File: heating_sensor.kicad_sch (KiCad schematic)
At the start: 3 parts

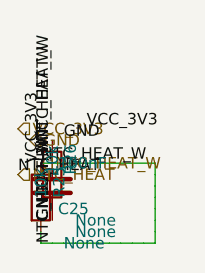
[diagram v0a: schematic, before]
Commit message: fix writer
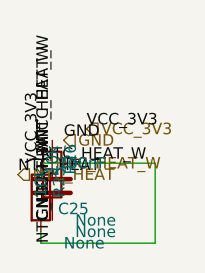
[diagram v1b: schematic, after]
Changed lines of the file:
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@@
 		(instances
 			(project "Untitled"
-				(path "/51987713-8abd-43cc-8dc0-832c464dab57"
+				(path "/c49ef74a-788a-4bab-9f15-e22212d1716d"
 					(reference "C25")
 					(unit 1)
@@
 		(instances
 			(project "Untitled"
-				(path "/51987713-8abd-43cc-8dc0-832c464dab57"
+				(path "/c49ef74a-788a-4bab-9f15-e22212d1716d"
 					(reference "R25")
 					(unit 1)
@@
 		(instances
 			(project "Untitled"
-				(path "/51987713-8abd-43cc-8dc0-832c464dab57"
+				(path "/c49ef74a-788a-4bab-9f15-e22212d1716d"
 					(reference "R26")
 					(unit 1)
@@
 	(wire
 		(pts
-			(xy 16.51 24.13) (xy 17.78 24.13)
-		)
-		(stroke
-			(width 0)
-			(type default)
-		)
-	)
-	(wire
-		(pts
-			(xy 17.78 24.13) (xy 19.05 24.13)
-		)
-		(stroke
-			(width 0)
-			(type default)
-		)
-	)
-	(wire
-		(pts
-			(xy 19.05 24.13) (xy 20.32 24.13)
-		)
-		(stroke
-			(width 0)
-			(type default)
-		)
-	)
-	(wire
-		(pts
-			(xy 20.32 24.13) (xy 21.59 24.13)
-		)
-		(stroke
-			(width 0)
-			(type default)
-		)
-	)
-	(wire
-		(pts
-			(xy 21.59 24.13) (xy 22.86 24.13)
-		)
-		(stroke
-			(width 0)
-			(type default)
-		)
-	)
-	(wire
-		(pts
-			(xy 22.86 24.13) (xy 24.13 24.13)
-		)
-		(stroke
-			(width 0)
-			(type default)
-		)
-	)
-	(wire
-		(pts
-			(xy 24.13 24.13) (xy 25.4 24.13)
-		)
-		(stroke
-			(width 0)
-			(type default)
-		)
-	)
-	(wire
-		(pts
-			(xy 25.4 24.13) (xy 26.67 24.13)
-		)
-		(stroke
-			(width 0)
-			(type default)
-		)
-	)
-	(wire
-		(pts
-			(xy 26.67 24.13) (xy 27.94 24.13)
-		)
-		(stroke
-			(width 0)
-			(type default)
-		)
-	)
-	(wire
-		(pts
-			(xy 27.94 24.13) (xy 29.21 24.13)
-		)
-		(stroke
-			(width 0)
-			(type default)
-		)
-	)
-	(wire
-		(pts
-			(xy 29.21 24.13) (xy 29.21 22.86)
-		)
-		(stroke
-			(width 0)
-			(type default)
-		)
-	)
-	(wire
-		(pts
-			(xy 29.21 22.86) (xy 29.21 21.59)
-		)
-		(stroke
-			(width 0)
-			(type default)
-		)
-	)
-	(wire
-		(pts
-			(xy 29.21 21.59) (xy 29.21 20.32)
-		)
-		(stroke
-			(width 0)
-			(type default)
-		)
-	)
-	(wire
-		(pts
-			(xy 29.21 20.32) (xy 29.21 19.05)
-		)
-		(stroke
-			(width 0)
-			(type default)
-		)
-	)
-	(wire
-		(pts
-			(xy 29.21 19.05) (xy 29.21 17.78)
-		)
-		(stroke
-			(width 0)
-			(type default)
-		)
-	)
-	(wire
-		(pts
-			(xy 29.21 17.78) (xy 29.21 16.51)
-		)
-		(stroke
-			(width 0)
-			(type default)
-		)
-	)
-	(wire
-		(pts
-			(xy 29.21 16.51) (xy 29.21 15.24)
+			(xy 16.51 24.13) (xy 29.21 24.13)
+		)
+		(stroke
+			(width 0)
+			(type default)
+		)
+	)
+	(wire
+		(pts
+			(xy 29.21 24.13) (xy 29.21 15.24)
 		)
 		(stroke
@@
 	(hierarchical_label "VCC_3V3"
 		(shape input)
-		(at 13.97 11.43 180)
+		(at 21.59 11.43 180)
 		(effects
 			(font
@@
 	(hierarchical_label "GND"
 		(shape input)
-		(at 15.24 12.7 180)
-		(effects
-			(font
+		(at 19.05 12.7 180)
+		(effects
+			(font
